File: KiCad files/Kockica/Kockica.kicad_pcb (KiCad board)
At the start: 2 copper layers, 26 x 26 mm, 4 parts, among them J1 Conn_01x02_Male, J2 Conn_01x02_Male, J3 Conn_01x02_Male, J4 Conn_01x02_Male

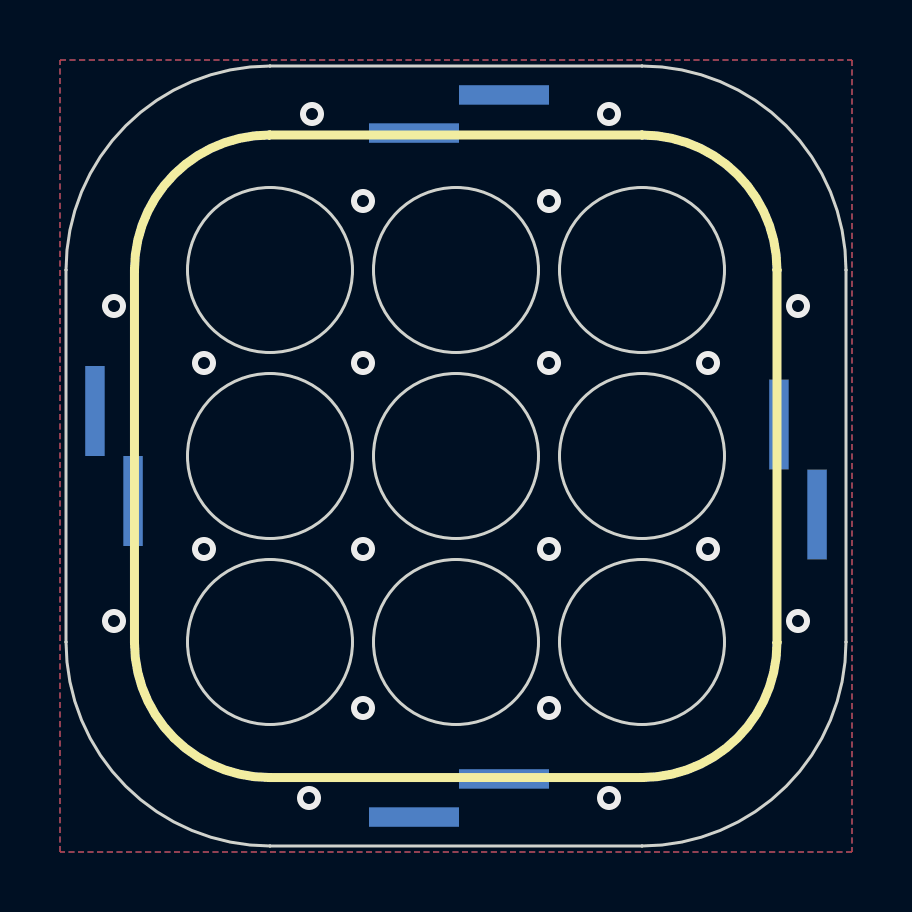
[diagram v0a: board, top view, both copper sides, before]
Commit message: update
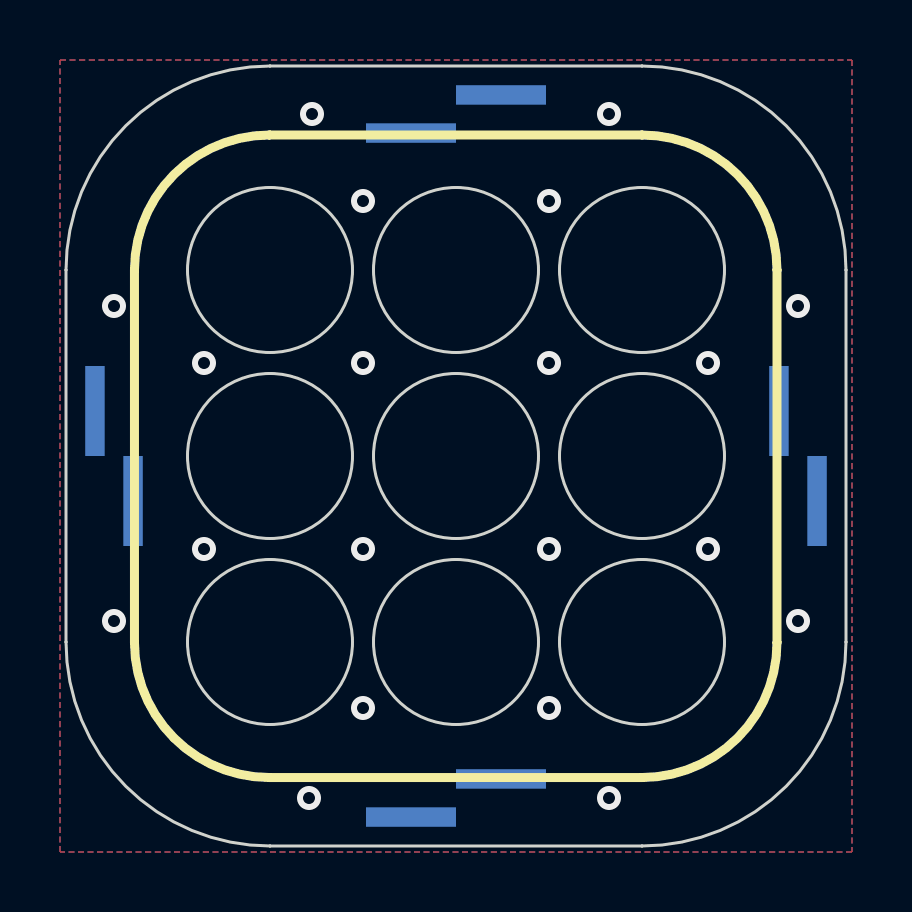
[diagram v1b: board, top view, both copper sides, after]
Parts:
- moved J4 0.45 mm to (67.6, 56.2)
- moved J1 0.10 mm to (56.2, 44.8)
- moved J3 0.10 mm to (56.2, 67.6)
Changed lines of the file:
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@@
   (net 1 "/TOUCHPAD")
   (footprint "Connector_PinHeader_1.27mm:PinHeader_1x02_P1.27mm_Vertical_SMD_Pin1Left" (layer "B.Cu")
-    (at 56.3 44.8)
+    (at 56.2 44.8)
     (descr "surface-mounted straight pin header, 1x02, 1.27mm pitch, single row, style 1 (pin 1 left)")
     (tags "Surface mounted pin header SMD 1x02 1.27mm single row style1 pin1 left")
@@
   )
   (footprint "Connector_PinHeader_1.27mm:PinHeader_1x02_P1.27mm_Vertical_SMD_Pin1Left" (layer "B.Cu")
-    (at 67.6 56.65 -90)
+    (at 67.6 56.2 -90)
     (descr "surface-mounted straight pin header, 1x02, 1.27mm pitch, single row, style 1 (pin 1 left)")
     (tags "Surface mounted pin header SMD 1x02 1.27mm single row style1 pin1 left")
@@
   )
   (footprint "Connector_PinHeader_1.27mm:PinHeader_1x02_P1.27mm_Vertical_SMD_Pin1Left" (layer "B.Cu")
-    (at 56.3 67.6 180)
+    (at 56.2 67.6 180)
     (descr "surface-mounted straight pin header, 1x02, 1.27mm pitch, single row, style 1 (pin 1 left)")
     (tags "Surface mounted pin header SMD 1x02 1.27mm single row style1 pin1 left")
@@
   (gr_line (start 62.4 69.2) (end 50 69.2) (layer "Edge.Cuts") (width 0.1))
   (gr_circle (center 62.4 50) (end 65.15 50) (layer "Edge.Cuts") (width 0.1) (fill none))
-  (gr_text "JLCJLCJLCJLC" (at 66.2 62.5 90) (layer "B.SilkS")
+  (gr_text "JLCJLCJLCJLC" (at 66.2 62.3 90) (layer "B.SilkS")
     (effects (font (size 0.9 0.9) (thickness 0.15)) (justify mirror))
   )
